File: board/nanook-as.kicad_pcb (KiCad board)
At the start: 2 copper layers, 75 x 42 mm, 43 parts, among them J1 Water Flow, J2 Address, J3 USB, J4 Conn_01x03, J5 Conn_01x03, J6 Conn_01x02, J7 Conn_01x02, J8 Conn_01x02, J9 Conn_01x02, U1 CD4051B, U2 ESP32-C3FN4, U3 LM1117MP-2.5, X1 I2C-6P, Y1 40MHz

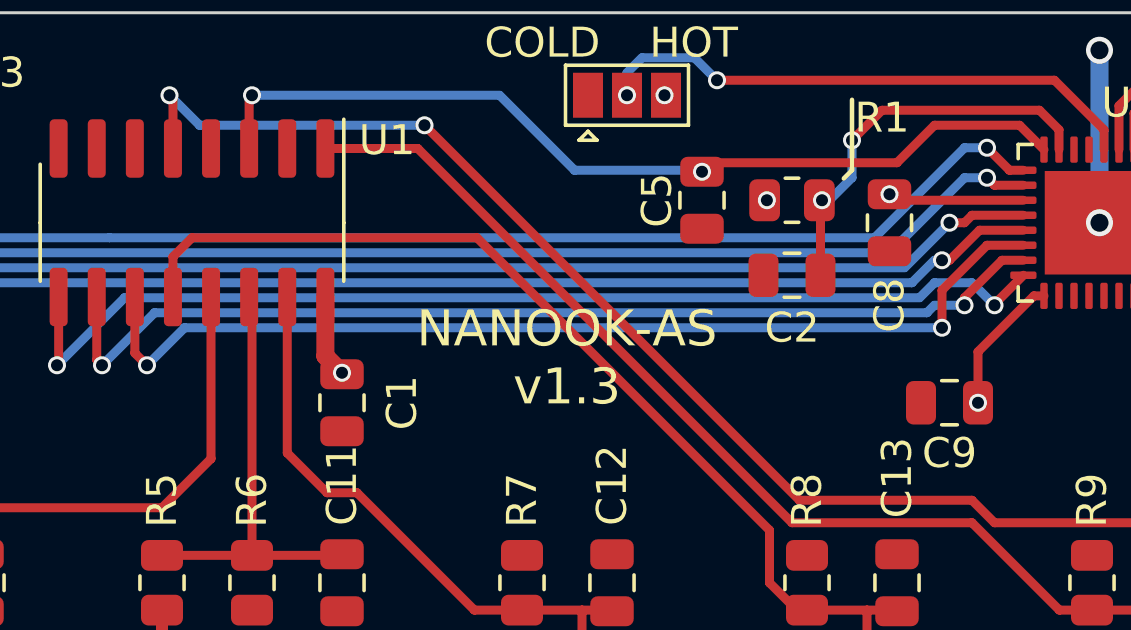
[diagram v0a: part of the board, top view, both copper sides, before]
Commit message: WIP
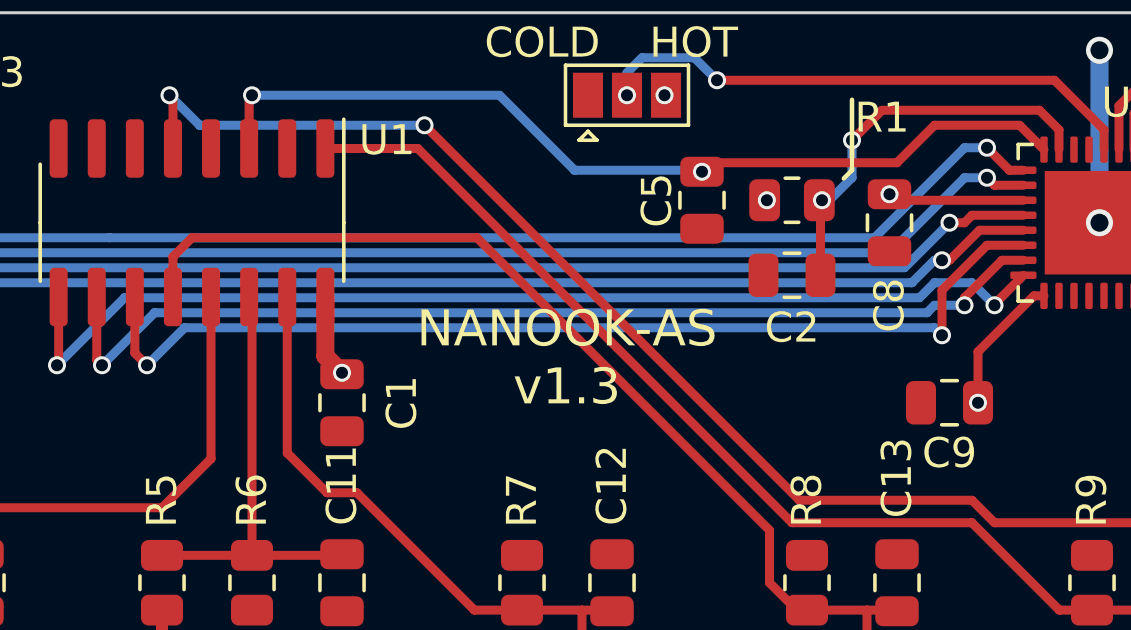
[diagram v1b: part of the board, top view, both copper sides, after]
